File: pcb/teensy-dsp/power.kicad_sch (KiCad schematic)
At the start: 0 parts

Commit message: update pcb layout
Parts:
- added C1, C2: 100u 16V, Capacitor_SMD:CP_Elec_6.3x5.9, symbol Device:C
- added J8: Barrel_Jack_Switch, Connector_BarrelJack:BarrelJack_CUI_PJ-102AH_Horizontal, symbol Connector:Barrel_Jack_Switch
- added U3: LM7805_TO220, Package_TO_SOT_SMD:SOT-223, symbol Regulator_Linear:LM7805_TO220
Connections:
- new net +5V: C2.1, U3.3 (VO)
- new net +9V: C1.1, J8.2, U3.1 (VI)
- new net GND: C1.2, C2.2, J8.1, U3.2 (GND)

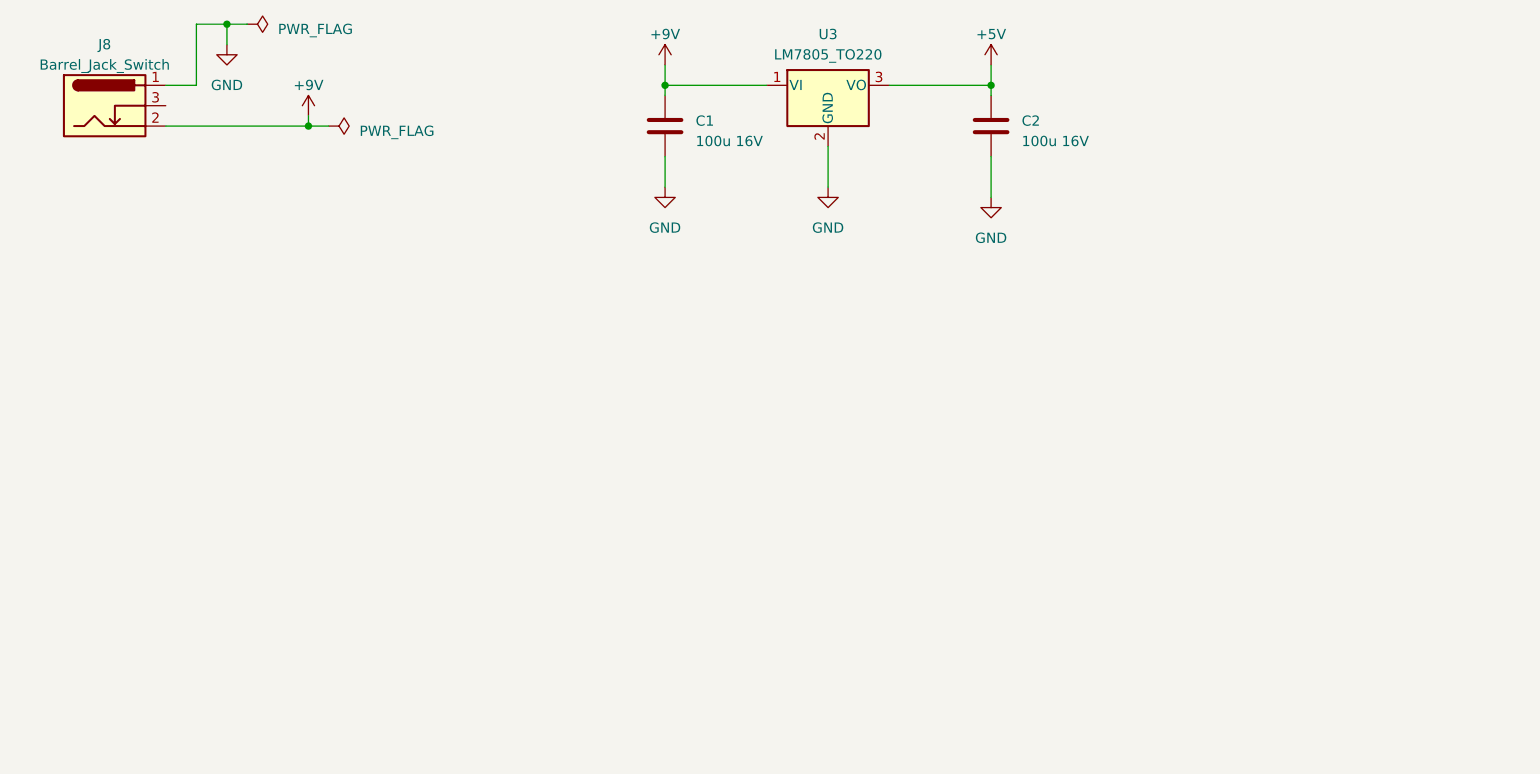
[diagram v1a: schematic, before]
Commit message: update pcb layout
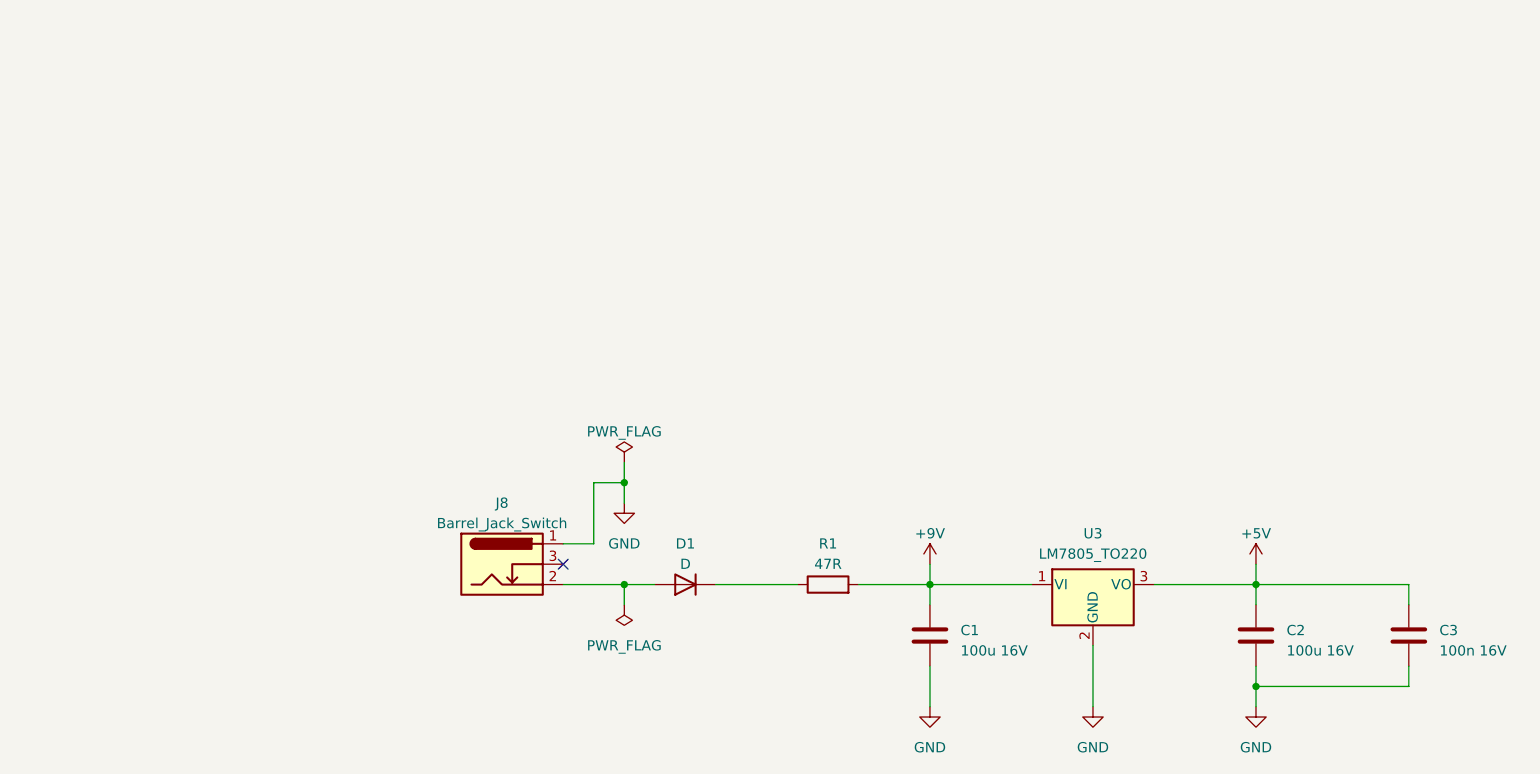
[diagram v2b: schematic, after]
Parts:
- added C3: 100n 16V, Capacitor_SMD:C_1210_3225Metric_Pad1.33x2.70mm_HandSolder, symbol Device:C
- added D1: D, Diode_THT:D_DO-41_SOD81_P10.16mm_Horizontal, symbol Device:D
- added R1: 47R, Resistor_SMD:R_1210_3225Metric_Pad1.30x2.65mm_HandSolder, symbol Device:R
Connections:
- net +5V: now also C3.1
- net +9V: now also R1.2; no longer J8.2
- net GND: now also C3.2
- new net: D1.1 (K), R1.1
- new net: D1.2 (A), J8.2
- no-connect marks 0 -> 1
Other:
- moved on the sheet: C1, C2, J8, U3
